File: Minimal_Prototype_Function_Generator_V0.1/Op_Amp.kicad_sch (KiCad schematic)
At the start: 27 parts, among them U1 ADA4817-2ACP

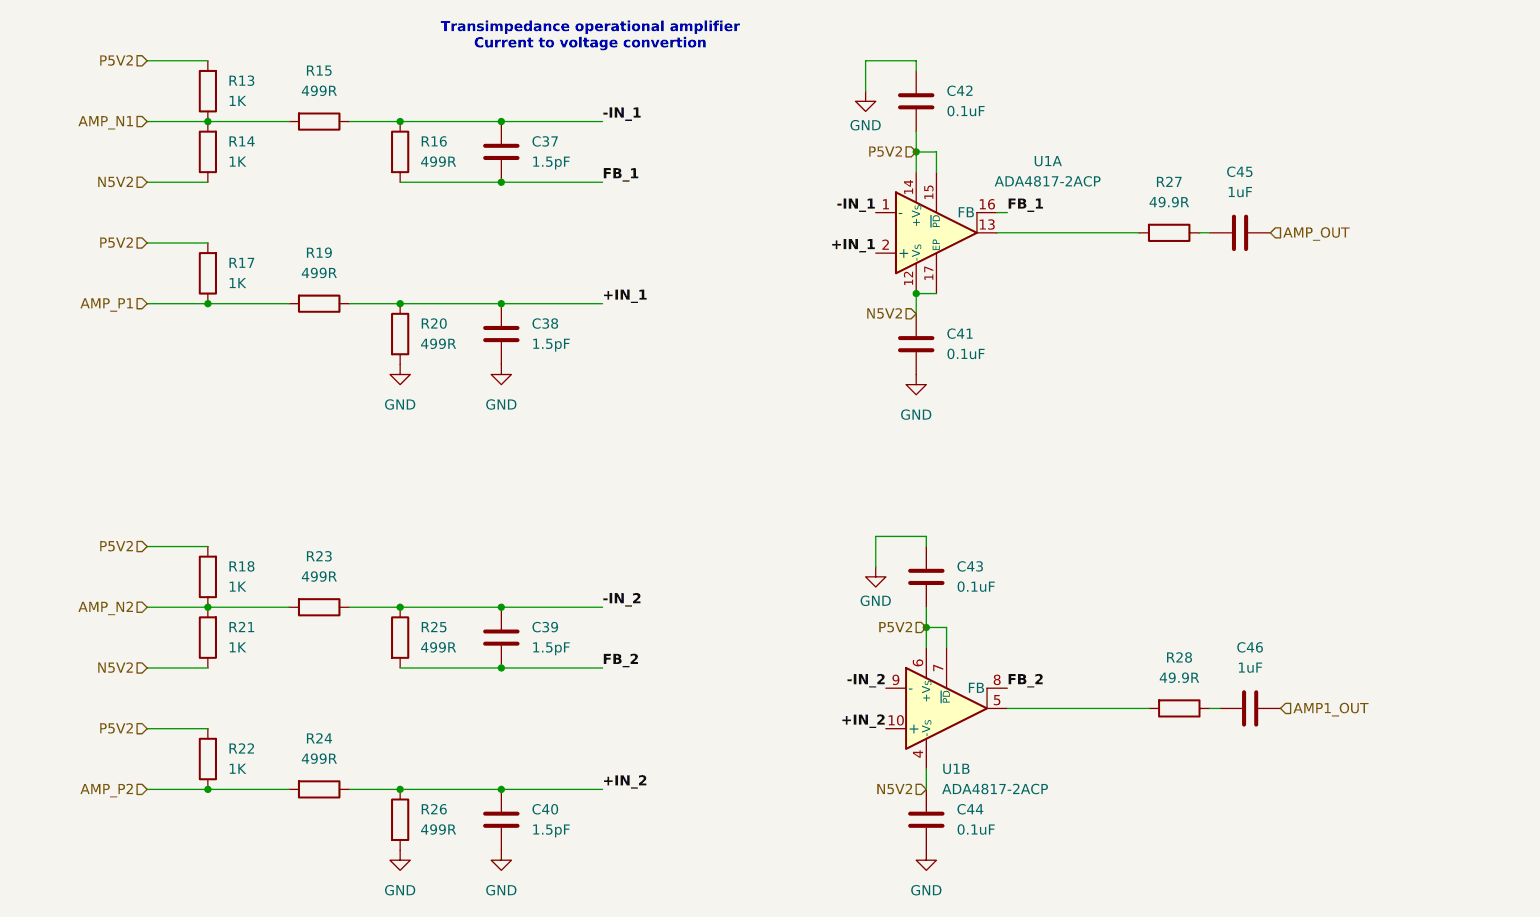
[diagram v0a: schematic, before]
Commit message: new pcb version
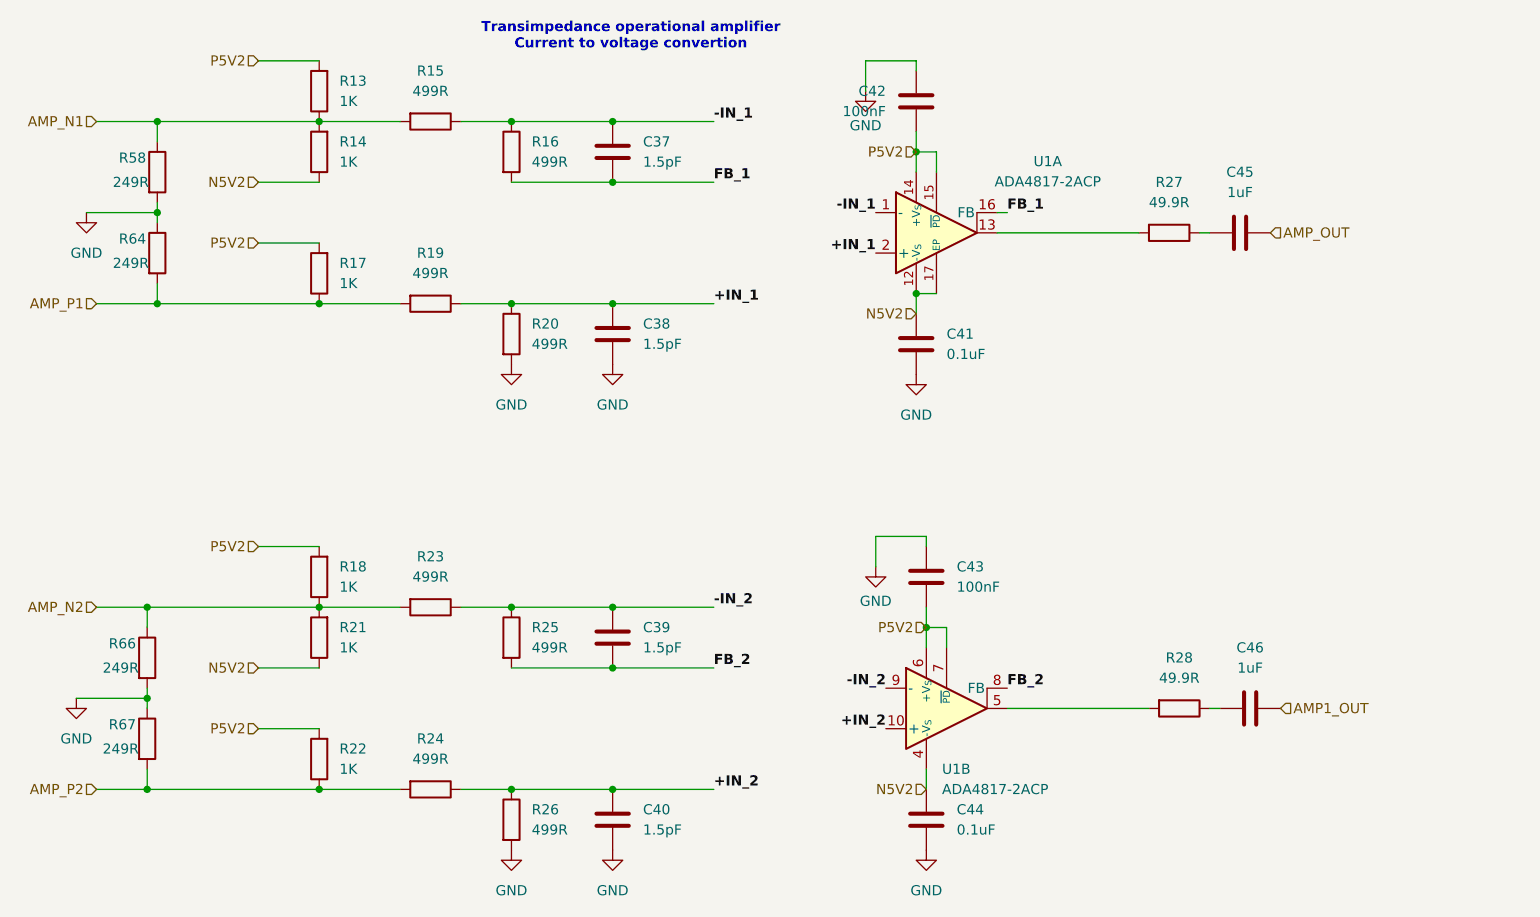
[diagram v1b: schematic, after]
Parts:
- added R58, R64, R66, R67: 249R, Insyte_Footprints:R_0603, symbol Device:R
- C37, C38, C39, C40, C41, C44, C45, C46: footprint Capacitor_SMD:C_0603_1608Metric -> Insyte_Footprints:C_0603
- C42, C43: value 0.1uF -> 100nF; footprint Capacitor_SMD:C_0603_1608Metric -> Insyte_Footprints:C_0603
- R13, R14, R15, R16, R17, R18, R19, R20, R21, R22, R23, R24, R25, R26, R27, R28: footprint Resistor_SMD:R_0603_1608Metric -> Insyte_Footprints:R_0603
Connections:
- net AMP_N1: now also R58.1
- net AMP_N2: now also R66.1
- net AMP_P1: now also R64.2
- net AMP_P2: now also R67.2
- net GND: now also R58.2, R64.1, R66.2, R67.1
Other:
- moved on the sheet: C37, C38, C39, C40, R13, R14, R15, R16, R17, R18, R19, R20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

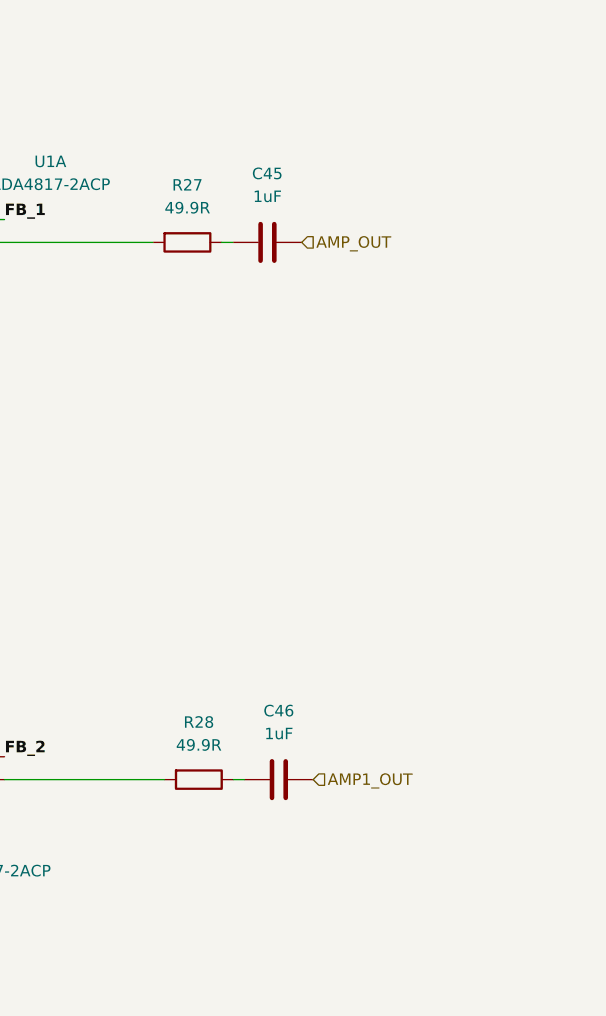
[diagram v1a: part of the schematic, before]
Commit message: V2.0
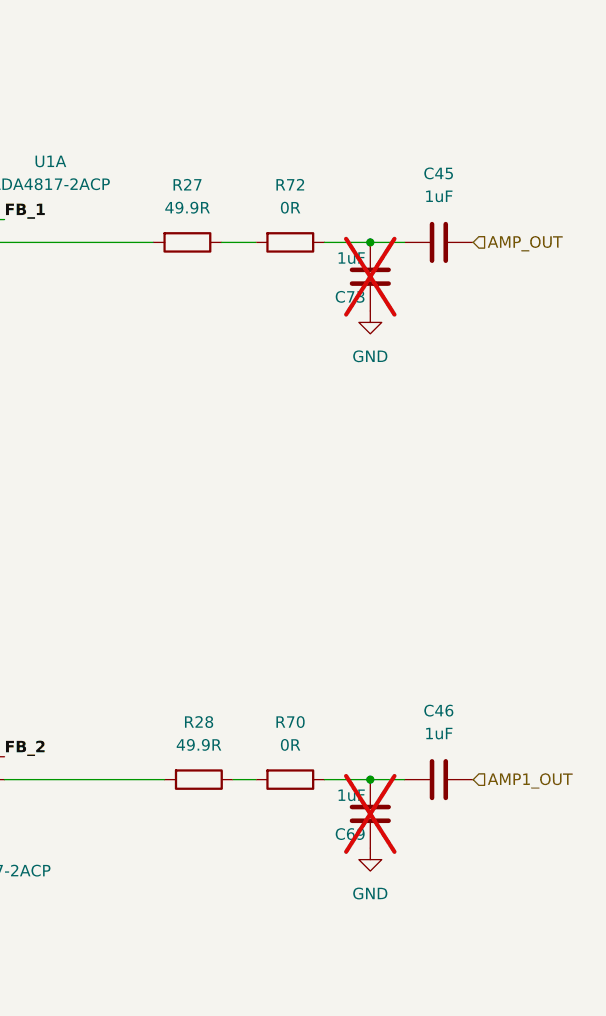
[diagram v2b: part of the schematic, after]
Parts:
- added C69, C73: 1uF, Insyte_Footprints:C_0603, symbol Device:C
- added R70, R72: 0R, Insyte_Footprints:R_0603, symbol Device:R
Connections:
- net GND: now also C69.2, C73.2
- net at C45.1: now also C73.1, R72.1; no longer R27.1
- net at C46.1: now also C69.1, R70.1; no longer R28.1
- new net: R28.1, R70.2
- new net: R27.1, R72.2
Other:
- moved on the sheet: C45, C46
